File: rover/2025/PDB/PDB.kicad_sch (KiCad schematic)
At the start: 66 parts, among them J1 USB_C_USB4105-GF-A, J2 ETH-CRJ036-5-TH, J3 TerminalBlock, SW1 TS09-63-25-WT-160-SMT-TR, SW2 TS09-63-25-WT-160-SMT-TR, U1 ESP32-S3-WROVER, U10 HSS-VN7140ASTR, U2 TVS, U3 SN65HVD232, U4 LDO-TLE4284DV33ATMA1, U5 XT60PW-M, U6 HSS-VN7004SLHTR, U7 HSS-VN7140ASTR, U8 HSS-VN7140ASTR, U9 HSS-VN7140ASTR

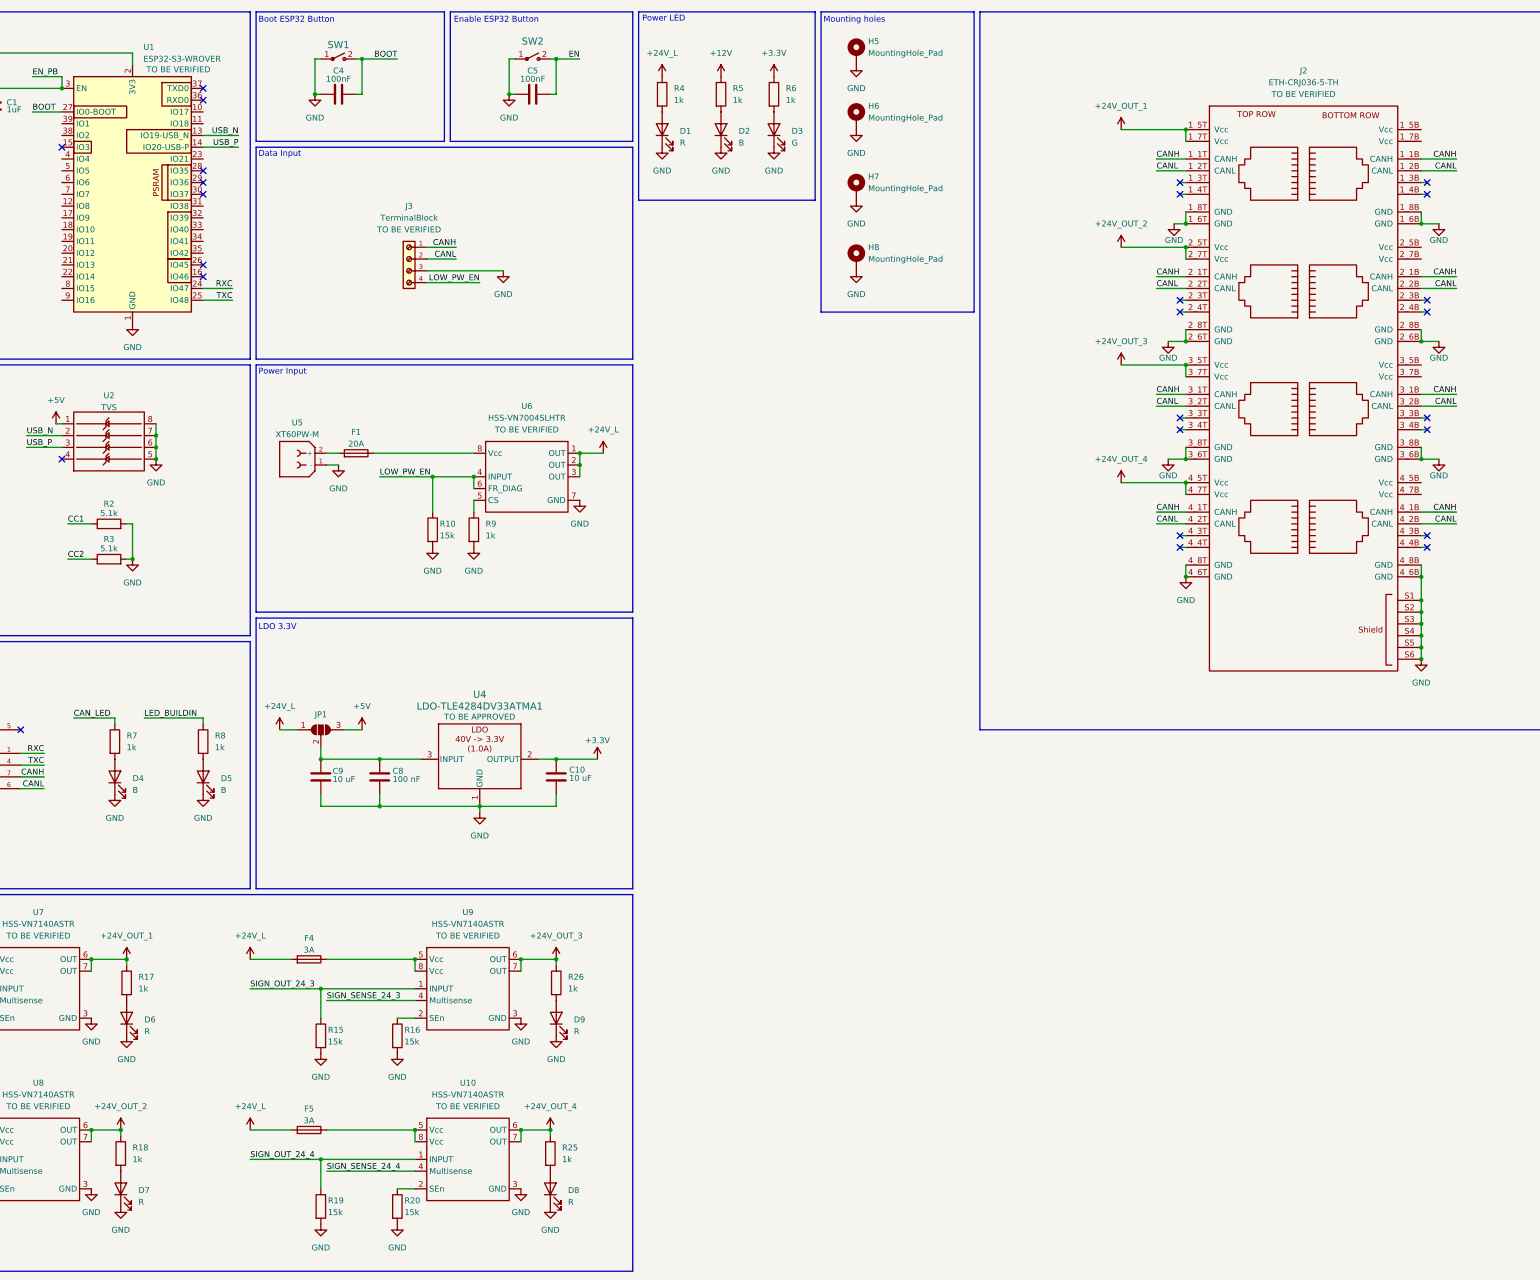
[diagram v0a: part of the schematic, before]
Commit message: .
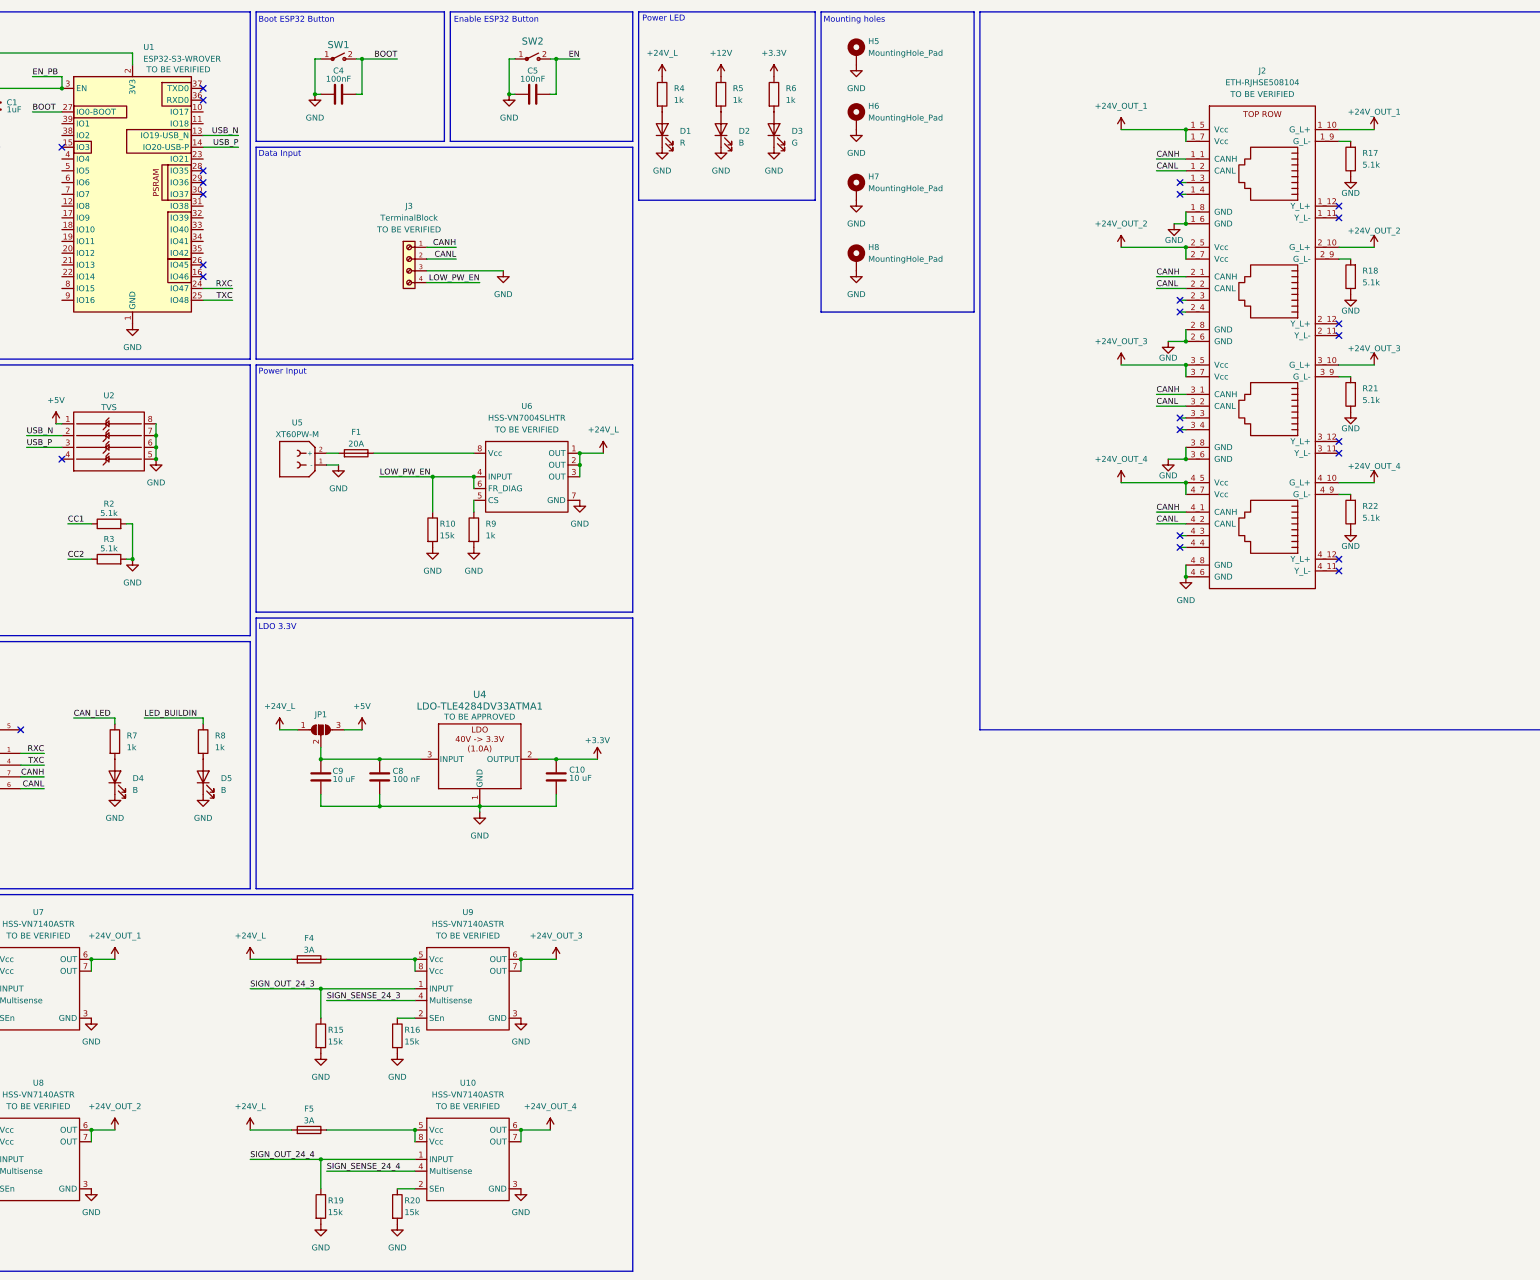
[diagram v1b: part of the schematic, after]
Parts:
- removed D6, D7, D8, D9: R, Diode_SMD:D_0805_2012Metric_Pad1.15x1.40mm_HandSolder, symbol Device:LED
- removed J2: ETH-CRJ036-5-TH, RoverFootprint:ETH-CRJ036-5-TH-2x4, symbol 0_RoverLibrary:ETH-CRJ036-5-TH
- removed R25, R26: 1k, Resistor_SMD:R_0805_2012Metric_Pad1.20x1.40mm_HandSolder, symbol Device:R
- added J2: ETH-RJHSE508104, RoverFootprint:ETH-RJHSE508104, symbol 0_RoverLibrary:ETH-RJHSE508104
- added R21, R22: 5.1k, Resistor_SMD:R_0805_2012Metric_Pad1.20x1.40mm_HandSolder, symbol Device:R
- R17, R18: value 1k -> 5.1k
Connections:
- net +24V_OUT_1: now also J2.1_10 (G_L+), J2.1_5 (Vcc), J2.1_7 (Vcc); no longer R17.1
- net +24V_OUT_2: now also J2.2_10 (G_L+), J2.2_5 (Vcc), J2.2_7 (Vcc); no longer R18.1
- net +24V_OUT_3: now also J2.3_10 (G_L+), J2.3_5 (Vcc), J2.3_7 (Vcc)
- net +24V_OUT_4: now also J2.4_10 (G_L+), J2.4_5 (Vcc), J2.4_7 (Vcc)
- net CANH: now also J2.1_1 (CANH), J2.2_1 (CANH), J2.3_1 (CANH), J2.4_1 (CANH)
- net CANL: now also J2.1_2 (CANL), J2.2_2 (CANL), J2.3_2 (CANL), J2.4_2 (CANL)
- net GND: now also R17.1, R18.1, J2.1_6 (GND), J2.1_8 (GND), J2.2_6 (GND), J2.2_8 (GND), J2.3_6 (GND), J2.3_8 (GND), J2.4_6 (GND), J2.4_8 (GND), R21.1, R22.1
- net at R17.2: now also J2.1_9 (G_L-)
- net at R18.2: now also J2.2_9 (G_L-)
- new net: J2.3_9 (G_L-), R21.2
- new net: J2.4_9 (G_L-), R22.2
